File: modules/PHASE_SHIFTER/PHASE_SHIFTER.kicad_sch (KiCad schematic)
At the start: 0 parts

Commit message: started phase shifter
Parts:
- added C1, C4: 470n, FormantKO:C_Rect, symbol FormantKO:C
- added C2: 4µ7, FormantKO:CP_Axial_600, symbol FormantKO:C_Polarized
- added C3: 1µ, FormantKO:C_Rect, symbol FormantKO:C
- added C5: 330n, FormantKO:C_Rect, symbol FormantKO:C
- added C6: 150n, FormantKO:C_Rect, symbol FormantKO:C
- added C7: 100n, FormantKO:C_Rect, symbol FormantKO:C
- added C8: 47n, FormantKO:C_Rect, symbol FormantKO:C
- added IC1, IC2: LM324, FormantKO:DIP-14, symbol FormantKO:LM324
- added P2: 50k, FormantKO:Potentiometer_Trimmer, symbol FormantKO:R_Trim
- added P4: 10k, FormantKO:PanelConnector_1x03, symbol FormantKO:R_Potentiometer
- added R1, R15, R16, R17, R18, R19, R2, R20: 100k, FormantKO:R_Axial_Horizontal, symbol FormantKO:R
- added R10, R11, R12, R13, R14, R21, R22, R3, R4, R5, R6, R7, R8, R9: 22k, FormantKO:R_Axial_Horizontal, symbol FormantKO:R
- added R23, R35: 10k, FormantKO:R_Axial_Horizontal, symbol FormantKO:R
- added S1: PHASING, FormantKO:PanelConnector_1x03, symbol FormantKO:SW_SPDT
- added T1, T2, T3, T4, T5, T6: N-FET, FormantKO:TO-92, symbol FormantKO:N-FET
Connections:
- new net: C4.1, IC1.14, R4.2, R5.1
- new net: IC1.2 (-), R5.2, R6.1
- new net: C5.1, IC1.1, R6.2, R7.1
- new net: C4.2, IC1.3 (+), R16.2, T2.3 (D)
- new net: C6.2, IC2.10 (+), R18.2, T4.3 (D)
- new net: P4.2, R22.1
- new net: IC2.6 (-), P2.3, R21.2, R22.2
- new net: C8.1, IC2.14, R12.2, R13.1
- new net: C8.2, IC2.3 (+), R20.2, T6.3 (D)
- new net: IC1.6 (-), R7.2, R8.1
- new net: T1.1 (G), T2.1 (G), T3.1 (G), T4.1 (G), T5.1 (G), T6.1 (G)
- new net: C5.2, IC1.5 (+), R17.2, T3.3 (D)
- new net: C3.2, IC1.12 (+), R15.2, T1.3 (D)
- new net: IC1.13 (-), R3.2, R4.1
- new net: C6.1, IC1.7, R8.2, R9.1
- new net: C3.1, IC1.8, R2.2, R3.1
- new net: IC2.7, R23.1, S1.1 (a)
- new net: C7.1, IC2.8, R10.2, R11.1
- new net: IC2.9 (-), R10.1, R9.2
- new net: IC2.1, P4.3, R14.2
- new net: IC2.2 (-), R13.2, R14.1
- new net: C1.2, IC1.10 (+), R1.2, R21.1, S1.3 (b)
- new net: C7.2, IC2.12 (+), R19.2, T5.3 (D)
- new net: IC2.13 (-), R11.2, R12.1
- new net: C2.1, S1.2 (c)
- new net: P2.1, P2.2, R23.2
- new net: IC1.9 (-), R2.1
- new net GND: IC2.5 (+), P4.1, R1.1, R15.1, R16.1, R17.1, R18.1, R19.1, R20.1, R35.1, T1.2 (S), T2.2 (S), T3.2 (S), T4.2 (S), T5.2 (S), T6.2 (S)
- new net IS: C1.1
- new net OS: C2.2, R35.2
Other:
- title: TEMPLATE -> PHASE-SHIFTER

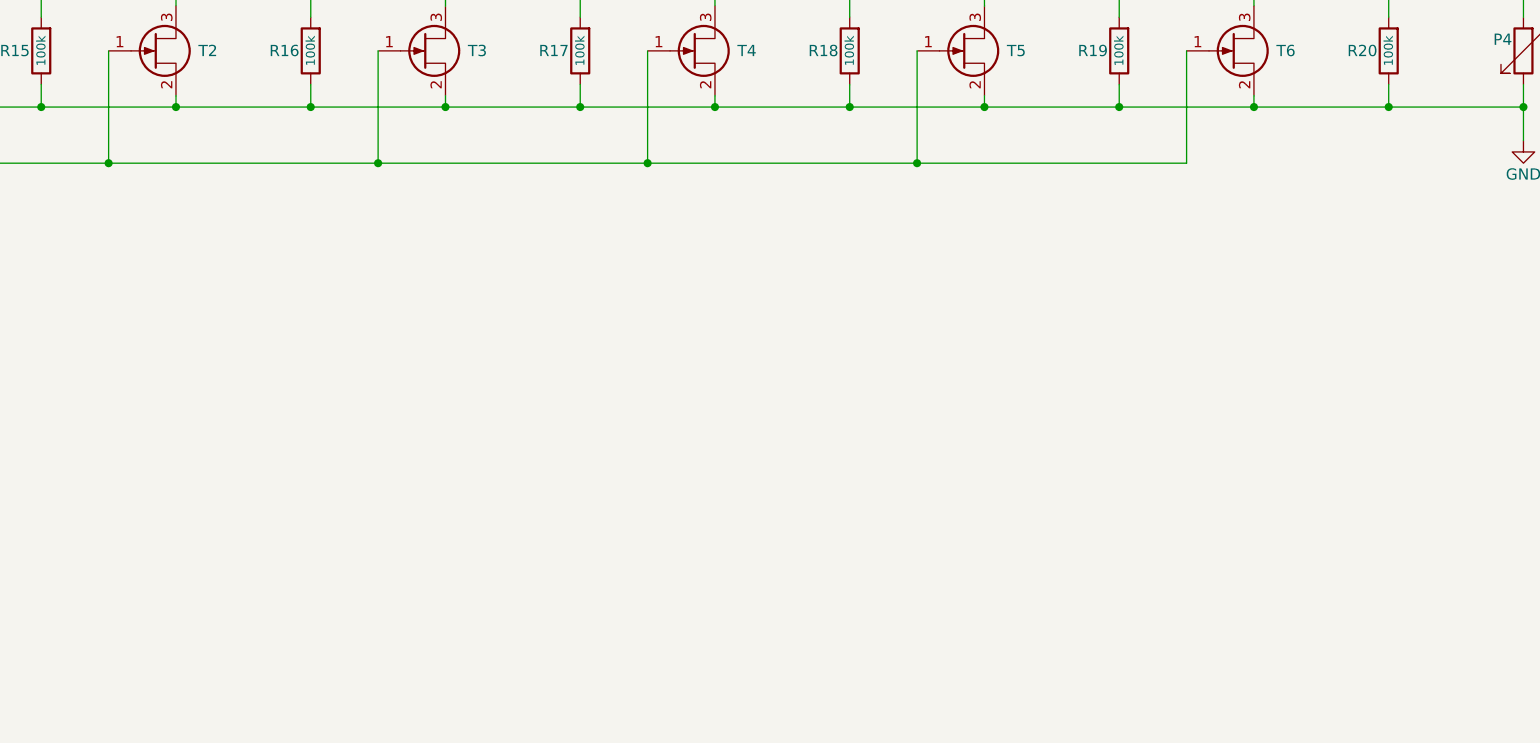
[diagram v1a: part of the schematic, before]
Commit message: phase shifter pcb placement
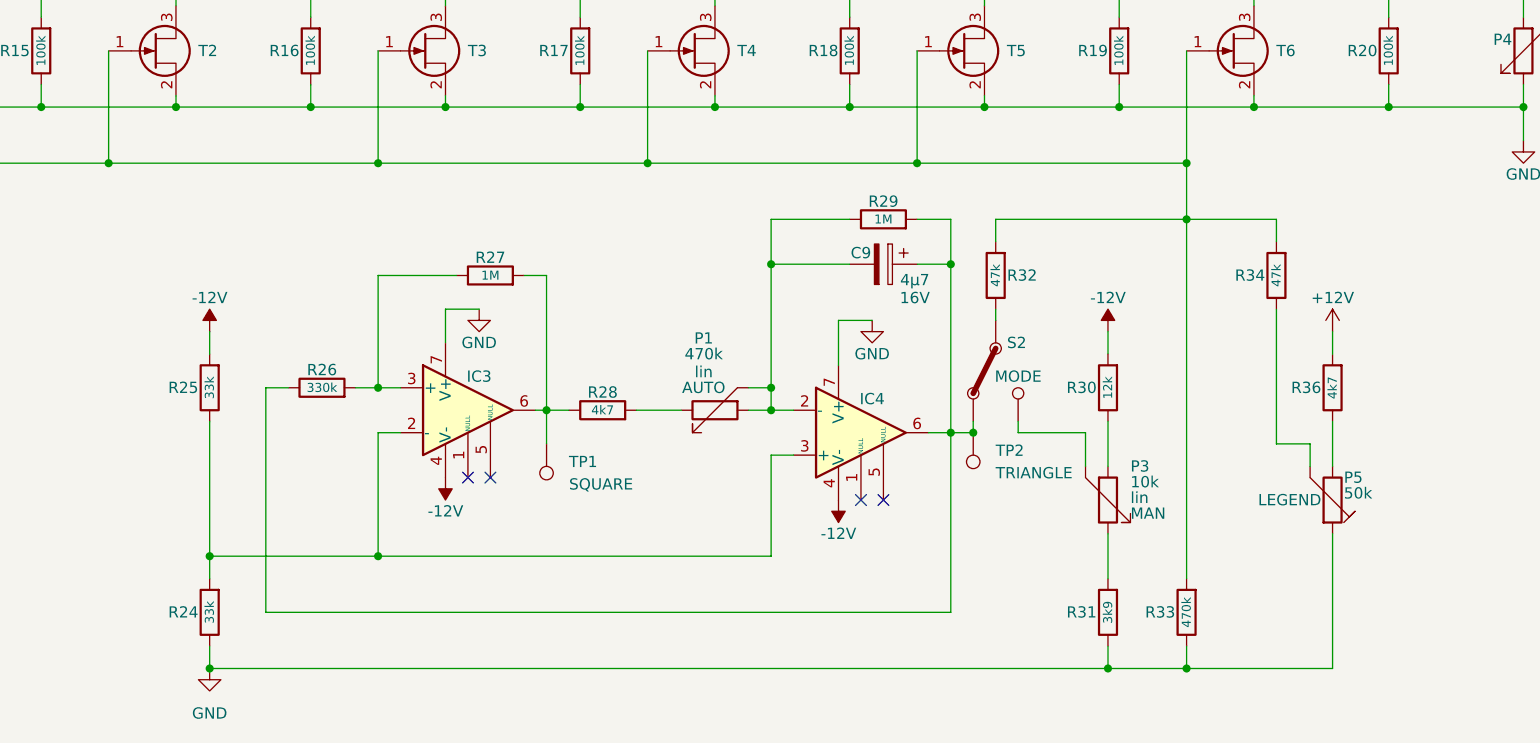
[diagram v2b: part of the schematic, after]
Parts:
- added C9: 4µ7, FormantKO:CP_Axial_600, symbol FormantKO:C_Polarized
- added IC3: OpAmp, FormantKO:DIP-8, symbol FormantKO:GenericOpAmp_Single_Swap
- added IC4: OpAmp, FormantKO:DIP-8, symbol FormantKO:GenericOpAmp_Single
- added P1: 470k, FormantKO:PanelConnector_1x03, symbol FormantKO:R_Potentiometer
- added P3: 10k, FormantKO:PanelConnector_1x03, symbol FormantKO:R_Potentiometer
- added P5: 50k, FormantKO:Potentiometer_Trimmer, symbol FormantKO:R_Trim
- added R24, R25: 33k, FormantKO:R_Axial_Horizontal, symbol FormantKO:R
- added R26: 330k, FormantKO:R_Axial_Horizontal, symbol FormantKO:R
- added R27, R29: 1M, FormantKO:R_Axial_Horizontal, symbol FormantKO:R
- added R28, R36: 4k7, FormantKO:R_Axial_Horizontal, symbol FormantKO:R
- added R30: 12k, FormantKO:R_Axial_Horizontal, symbol FormantKO:R
- added R31: 3k9, FormantKO:R_Axial_Horizontal, symbol FormantKO:R
- added R32, R34: 47k, FormantKO:R_Axial_Horizontal, symbol FormantKO:R
- added R33: 470k, FormantKO:R_Axial_Horizontal, symbol FormantKO:R
- added S2: MODE, FormantKO:PanelConnector_1x03, symbol FormantKO:SW_SPDT
- added TP1: SQUARE, TestPoint:TestPoint_Loop_D2.50mm_Drill1.0mm, symbol Connector:TestPoint
- added TP2: TRIANGLE, TestPoint:TestPoint_Loop_D2.50mm_Drill1.0mm, symbol Connector:TestPoint
- C4, C5, C6, C7, C8: footprint FormantKO:C_Rect -> FormantKO:C_Rect_300_400
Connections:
- net GND: now also IC3.7 (V+), IC4.7 (V+), P5.3, R24.1, R31.1, R33.1
- net at T1.1 (G), T2.1 (G), T3.1 (G)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: now also R32.2, R33.2, R34.2
- new net: IC3.6, R27.2, R28.1, TP1.1
- new net: P3.1, R31.2
- new net: C9.2, IC4.2 (-), P1.2, P1.3, R29.1
- new net: IC3.2 (-), IC4.3 (+), R24.2, R25.1
- new net: C9.1, IC4.6, R26.1, R29.2, S2.1 (a), TP2.1
- new net: P3.2, S2.3 (b)
- new net: P3.3, R30.1
- new net: P1.1, R28.2
- new net: R32.1, S2.2 (c)
- new net: P5.1, R36.1
- new net: P5.2, R34.1
- new net: IC3.3 (+), R26.2, R27.1
- new net +12V: R36.2
- new net -12V: IC3.4 (V-), IC4.4 (V-), R25.2, R30.2
- no-connect marks 0 -> 4
